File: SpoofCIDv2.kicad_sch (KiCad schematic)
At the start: 28 parts, among them J1 Micro_SD_Card, J2 Conn_01x08, J3 Conn_01x04_Pin, J4 Conn_01x03_Pin, J5 Conn_01x05_Pin, J6 Conn_01x02_Pin, U1 TS3A27518EPW, U2 CY8C4245LQI-483, U3 TVS0500DRV

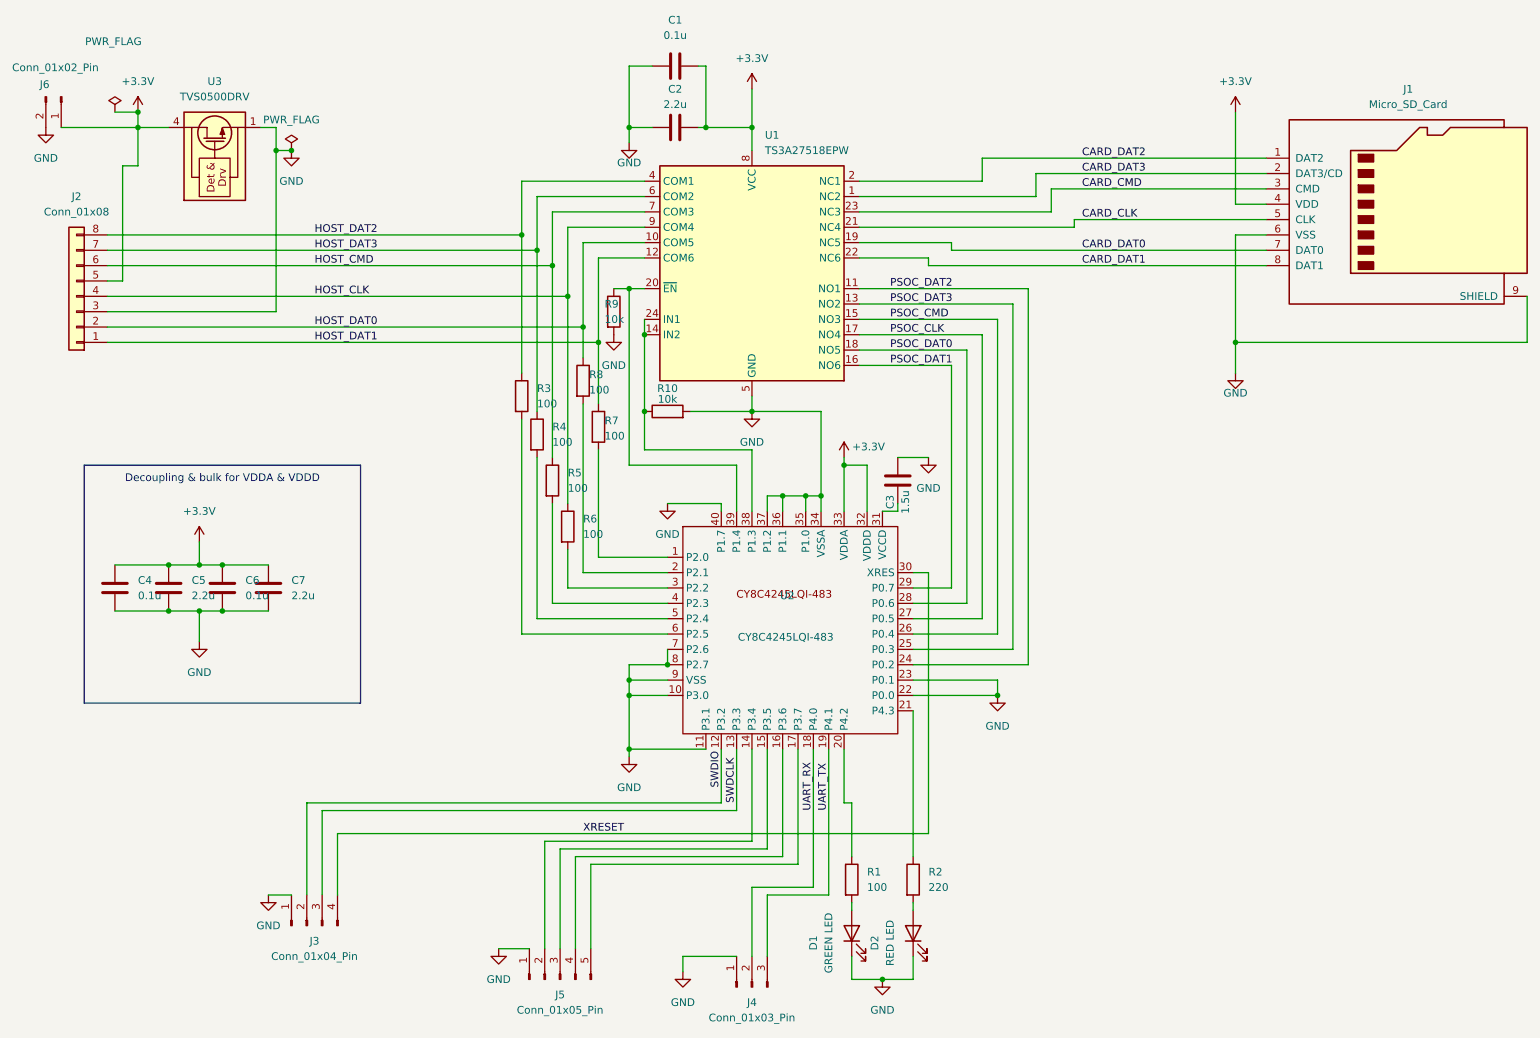
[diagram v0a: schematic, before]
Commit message: Modified PCB final version
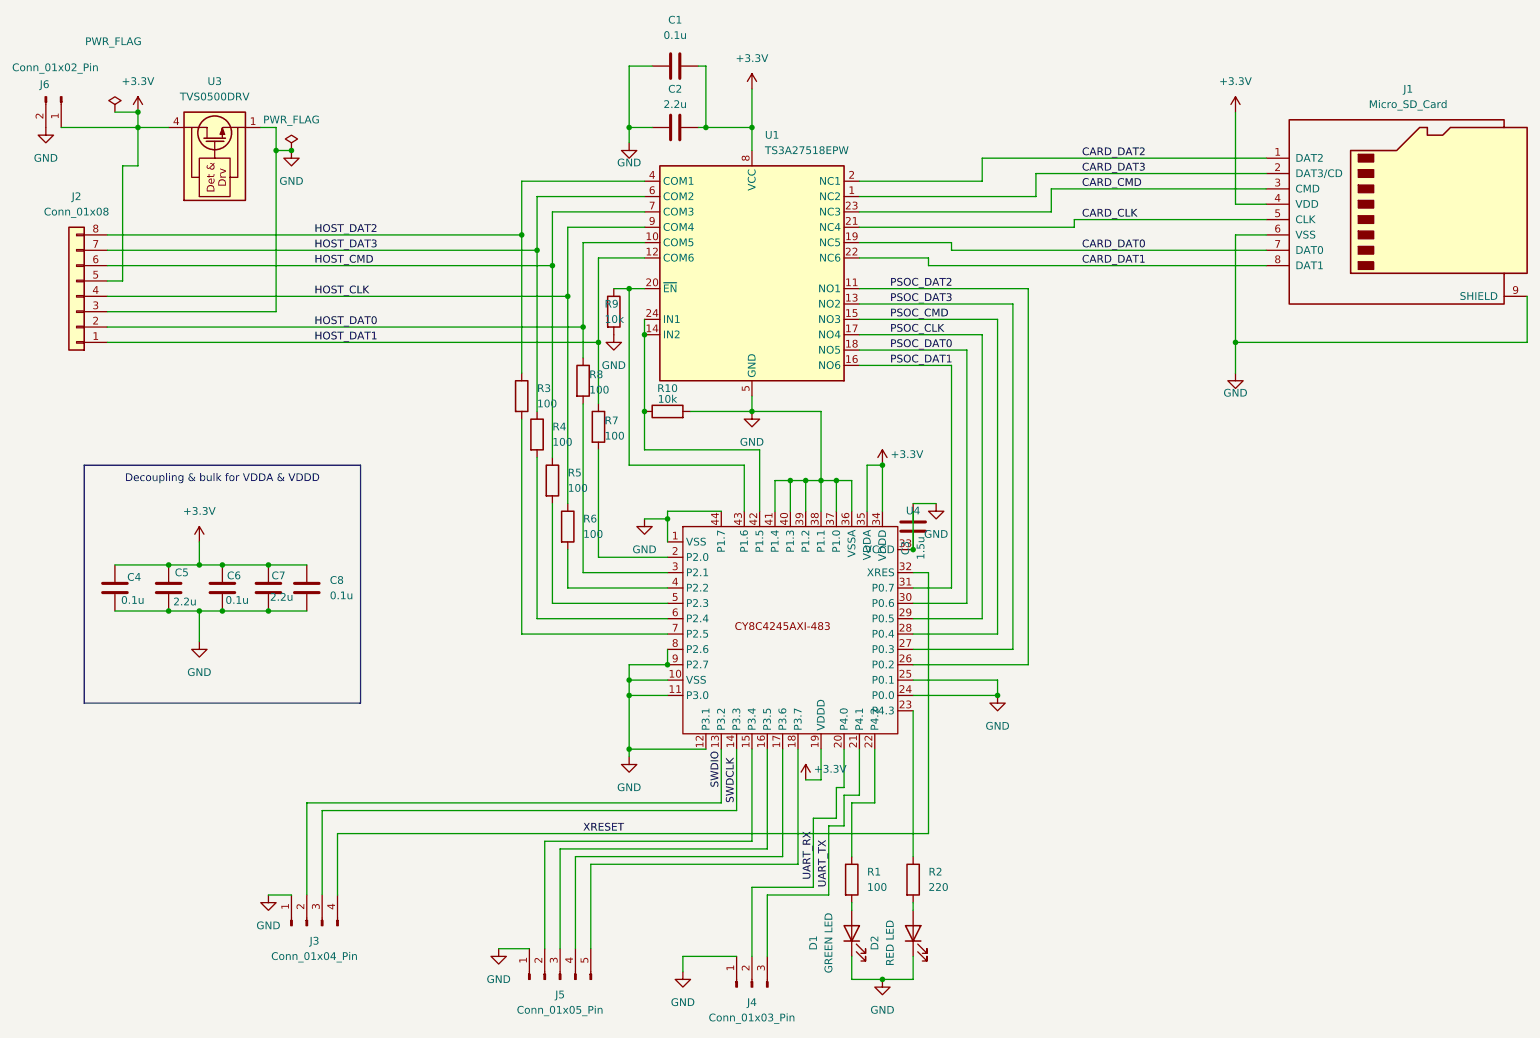
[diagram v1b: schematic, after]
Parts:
- removed U2: CY8C4245LQI-483, Package_DFN_QFN:QFN-40-1EP_6x6mm_P0.5mm_EP4.6x4.6mm, symbol Libreria:CY8C4245LQI-483
- added C8: 0.1u, Capacitor_SMD:C_0402_1005Metric, symbol Device:C
- added U4: ~, Package_QFP:TQFP-44_10x10mm_P0.8mm, symbol Libreria:CY8C4245AXI-483
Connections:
- net +3.3V: now also C8.2, U4.19 (VDDD), U4.34 (VDDD), U4.35 (VDDA)
- net GND: now also C8.1, U4.1 (VSS), U4.10 (VSS), U4.11 (P3.0), U4.12 (P3.1), U4.24 (P0.0), U4.25 (P0.1), U4.36 (VSSA), U4.37 (P1.0), U4.38 (P1.1), U4.39 (P1.2), U4.40 (P1.3), U4.41 (P1.4), U4.44 (P1.7), U4.8 (P2.6), U4.9 (P2.7)
- net PSOC_CLK: now also U4.29 (P0.5)
- net PSOC_CMD: now also U4.28 (P0.4)
- net PSOC_DAT0: now also U4.30 (P0.6)
- net PSOC_DAT1: now also U4.31 (P0.7)
- net PSOC_DAT2: now also U4.26 (P0.2)
- net PSOC_DAT3: now also U4.27 (P0.3)
- net SWDCLK: now also U4.14 (P3.3)
- net SWDIO: now also U4.13 (P3.2)
- net UART_RX: now also U4.20 (P4.0)
- net UART_TX: now also U4.21 (P4.1)
- net XRESET: now also U4.32 (XRES)
- net at R3.2: now also U4.7 (P2.5)
- net at R5.2: now also U4.5 (P2.3)
- net at J5.2 (Pin_2): now also U4.15 (P3.4)
- net at J5.3 (Pin_3): now also U4.16 (P3.5)
- net at J5.4 (Pin_4): now also U4.17 (P3.6)
- net at J5.5 (Pin_5): now also U4.18 (P3.7)
- net at R4.2: now also U4.6 (P2.4)
- net at R7.2: now also U4.2 (P2.0)
- net at R8.2: now also U4.3 (P2.1)
- net at R1.1: now also U4.22 (P4.2)
- net at R2.1: now also U4.23 (P4.3)
- net at R6.2: now also U4.4 (P2.2)
- net at C3.1: now also U4.33 (VCCD)
- net at R10.1, U1.14 (IN2), U1.24 (IN1): now also U4.42 (P1.5)
- net at R9.1, U1.20 (~{EN}): now also U4.43 (P1.6)
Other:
- moved on the sheet: C3
